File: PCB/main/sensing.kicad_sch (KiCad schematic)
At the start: 4 parts, among them U1 LM61BIZ/NOPD_TempSensor(TO-92), U2 LPS22HBTR_Barometer

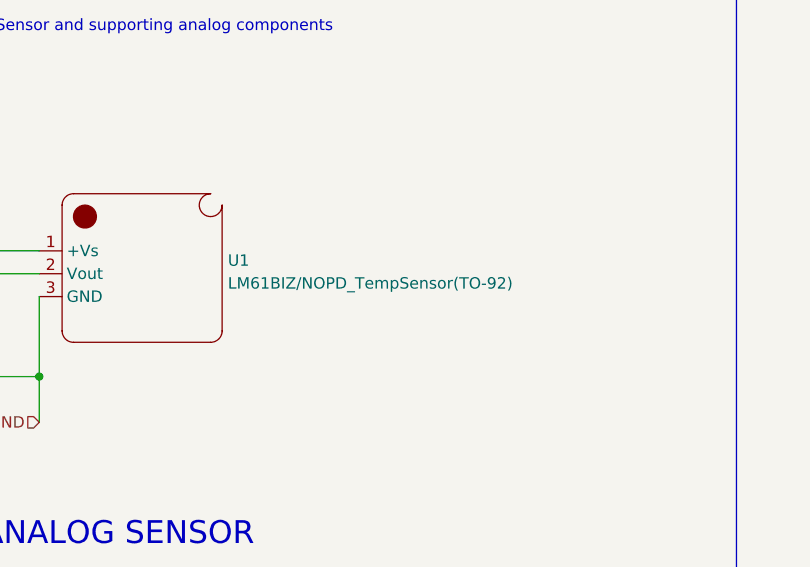
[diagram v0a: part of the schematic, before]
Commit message: Updated footprints
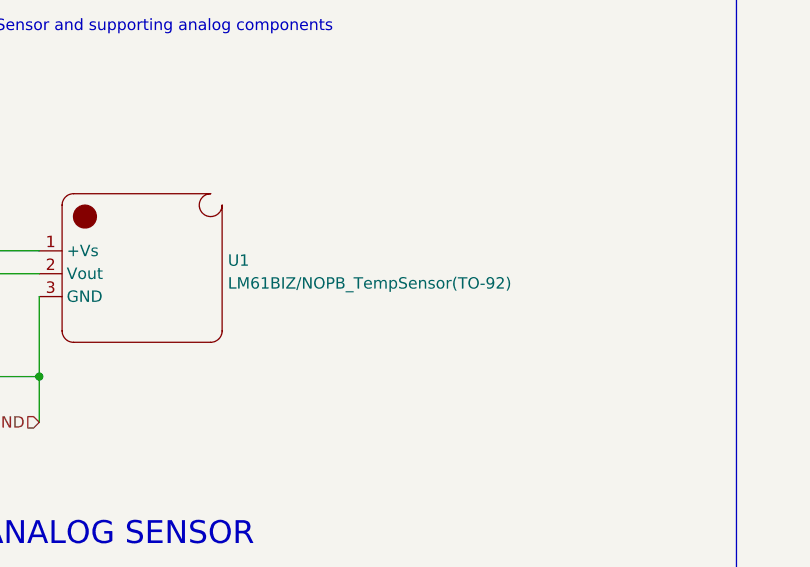
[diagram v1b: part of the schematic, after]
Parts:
- removed U1: LM61BIZ/NOPD_TempSensor(TO-92), EEE3088F_Footprints:TO-92-3_L4.9-W3.7-P1.27-L, symbol AAA 3088F:TO-92_Temperature_Sensor
- removed U2: LPS22HBTR_Barometer, EEE3088F_Footprints:QFN50P210X200X80-10N, symbol AAA 3088F:_C94049_Barometer
- added U1: LM61BIZ/NOPB_TempSensor(TO-92), EEE3088F_Footprints:TO-92-3_L4.9-W3.7-P1.27-L, symbol AAA_3088F:LM61BIZ/NOPB_TempSensor(TO-92)
- added U2: LPS22HBTR_Barometer, EEE3088F_Footprints:QFN50P210X200X80-10N, symbol AAA_3088F: LPS22HBTR_Barometer
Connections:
- net BARO_LSB: now also U2.5 (SDO/SA0)
- net BARO_SCL: now also U2.2 (SCL/SPC)
- net BARO_SDA: now also U2.4 (SDA/SDI/SDO)
- net BARO_VDD: now also U2.10 (VDD)
- net COMM: now also U2.1 (VDD_IO), U2.6 (CS)
- net GND: now also U1.3 (GND), U2.3 (RES), U2.8 (GND), U2.9 (GND)
- net TEMP_OUT: now also U1.2 (Vout)
- net TEMP_VCC: now also U1.1 (+Vs)
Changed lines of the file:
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@@
     (effects (font (size 1.27 1.27)) (justify right))
   )
-  (symbol (lib_id "AAA 3088F:TO-92_Temperature_Sensor") (at 73.66 46.99 0) (unit 1)
-    (in_bom yes) (on_board yes) (fields_autoplaced)
-    (property "Reference" "U1" (id 0) (at 83.1851 45.5203 0)
-      (effects (font (size 1.27 1.27)) (justify left))
-    )
-    (property "Value" "LM61BIZ/NOPD_TempSensor(TO-92)" (id 1) (at 83.1851 48.0572 0)
-      (effects (font (size 1.27 1.27)) (justify left))
-    )
-    (property "Footprint" "EEE3088F_Footprints:TO-92-3_L4.9-W3.7-P1.27-L" (id 2) (at 73.66 46.99 0)
-      (effects (font (size 1.27 1.27)) hide)
-    )
-    (property "Datasheet" "" (id 3) (at 73.66 46.99 0)
-      (effects (font (size 1.27 1.27)) hide)
-    )
-    (pin "1")
-    (pin "2")
-    (pin "3")
-  )
-  (symbol (lib_id "AAA 3088F:_C94049_Barometer") (at 207.01 54.61 0) (unit 1)
+  (symbol (lib_id "AAA_3088F: LPS22HBTR_Barometer") (at 207.01 54.61 0) (unit 1)
     (in_bom yes) (on_board yes) (fields_autoplaced)
     (property "Reference" "U2" (id 0) (at 207.01 37.0671 0))
-    (property "Value" "LPS22HBTR_Barometer" (id 1) (at 207.01 39.604 0))
+    (property "Value" " LPS22HBTR_Barometer" (id 1) (at 207.01 39.604 0))
     (property "Footprint" "EEE3088F_Footprints:QFN50P210X200X80-10N" (id 2) (at 207.01 54.61 0)
       (effects (font (size 1.27 1.27)) hide)
@@
     (pin "9")
   )
+  (symbol (lib_id "AAA_3088F:LM61BIZ{slash}NOPB_TempSensor(TO-92)") (at 73.66 46.99 0) (unit 1)
+    (in_bom yes) (on_board yes) (fields_autoplaced)
+    (property "Reference" "U1" (id 0) (at 83.1851 45.5203 0)
+      (effects (font (size 1.27 1.27)) (justify left))
+    )
+    (property "Value" "LM61BIZ/NOPB_TempSensor(TO-92)" (id 1) (at 83.1851 48.0572 0)
+      (effects (font (size 1.27 1.27)) (justify left))
+    )
+    (property "Footprint" "EEE3088F_Footprints:TO-92-3_L4.9-W3.7-P1.27-L" (id 2) (at 73.66 46.99 0)
+      (effects (font (size 1.27 1.27)) hide)
+    )
+    (property "Datasheet" "" (id 3) (at 73.66 46.99 0)
+      (effects (font (size 1.27 1.27)) hide)
+    )
+    (pin "1")
+    (pin "2")
+    (pin "3")
+  )
   (symbol (lib_id "Device:C_Polarized_Small_US") (at 50.8 52.07 0) (unit 1)

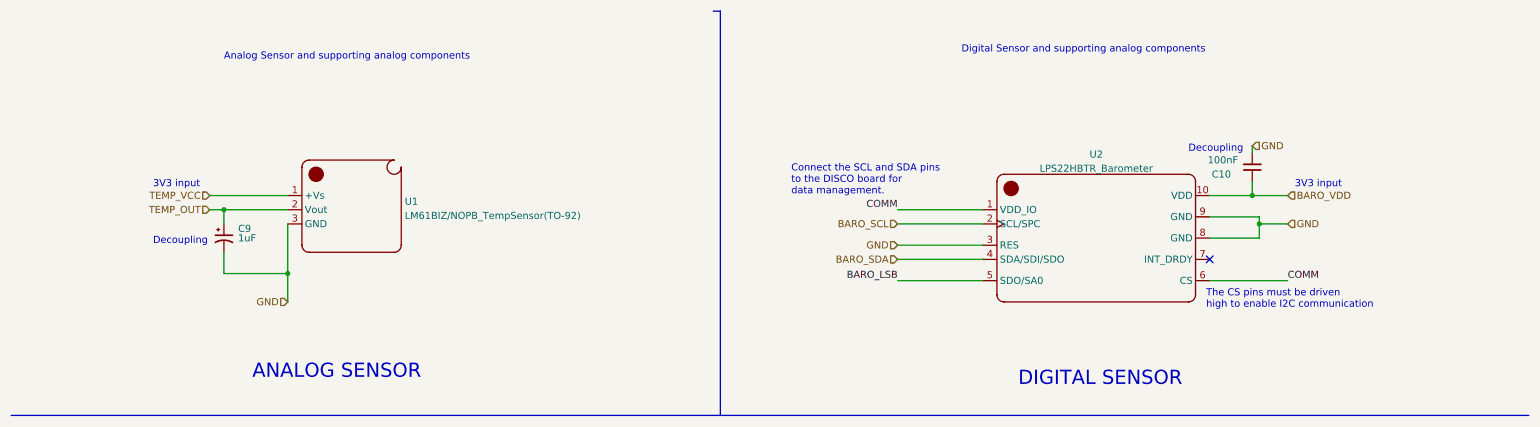
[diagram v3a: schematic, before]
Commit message: Finished Gerbers and updated BOM
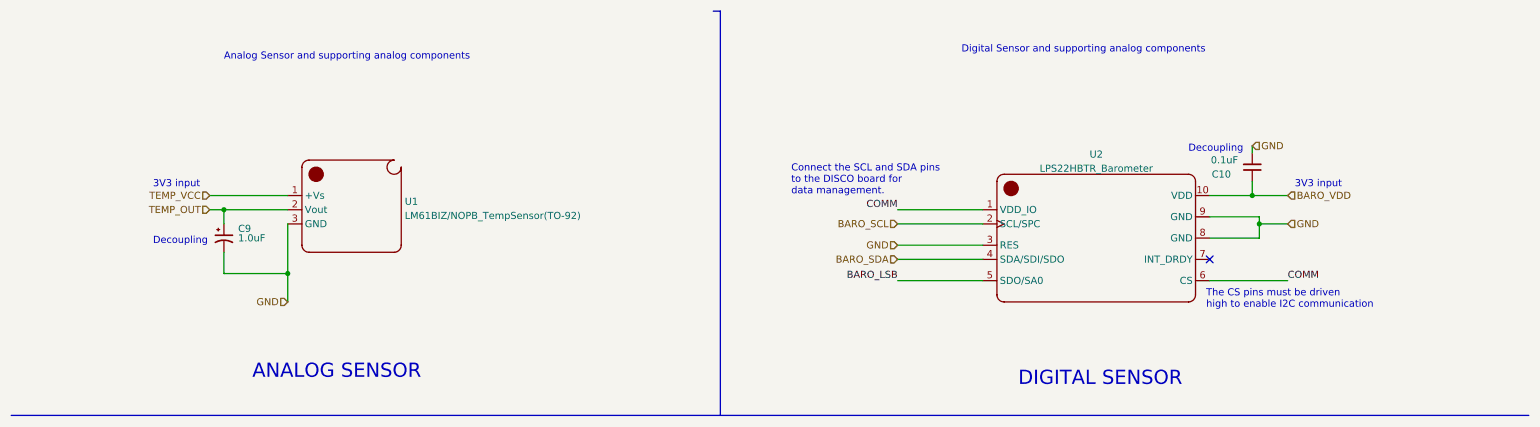
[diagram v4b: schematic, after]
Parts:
- C10: value 100nF -> 0.1uF; LCSC (none) -> C1525
- C9: value 1uF -> 1.0uF; LCSC (none) -> C15849
- U1: LCSC (none) -> C90846
- U2: LCSC (none) -> C94049
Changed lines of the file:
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@@
+      (effects (font (size 1.27 1.27)) hide)
+    )
+    (property "LCSC" "C94049" (id 4) (at 207.01 54.61 0)
       (effects (font (size 1.27 1.27)) hide)
     )
@@
       (effects (font (size 1.27 1.27)) hide)
     )
+    (property "LCSC" "C90846" (id 4) (at 73.66 46.99 0)
+      (effects (font (size 1.27 1.27)) hide)
+    )
     (pin "1")
     (pin "2")
@@
       (effects (font (size 1.27 1.27)) (justify left))
     )
-    (property "Value" "1uF" (id 1) (at 53.34 52.07 0)
+    (property "Value" "1.0uF" (id 1) (at 53.34 52.07 0)
       (effects (font (size 1.27 1.27)) (justify left))
     )
@@
     )
     (property "Datasheet" "~" (id 3) (at 50.8 52.07 0)
+      (effects (font (size 1.27 1.27)) hide)
+    )
+    (property "LCSC" "C15849" (id 4) (at 50.8 52.07 0)
       (effects (font (size 1.27 1.27)) hide)
     )
@@
       (effects (font (size 1.27 1.27)) (justify left))
     )
-    (property "Value" "100nF" (id 1) (at 232.41 38.0938 0)
+    (property "Value" "0.1uF" (id 1) (at 232.41 38.0938 0)
       (effects (font (size 1.27 1.27)) (justify left))
     )
@@
       (effects (font (size 1.27 1.27)) hide)
     )
+    (property "LCSC" "C1525" (id 4) (at 234.95 39.37 0)
+      (effects (font (size 1.27 1.27)) hide)
+    )
